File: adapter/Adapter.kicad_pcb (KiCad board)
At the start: 4 copper layers, 54 parts, among them J1 USB_B_Micro, J2 2040210-1, J3 USB_C_Receptacle, J4 Conn_01x05_Male, J5 Conn_01x03_Male, Q1 IRLML2244TRPBF, SW1 BOOT, SW2 BOOT, U1 SN75DP119RGYT, U2 LD1117S33TR, U3 STM32F072C8Tx, Y1 8MHZ

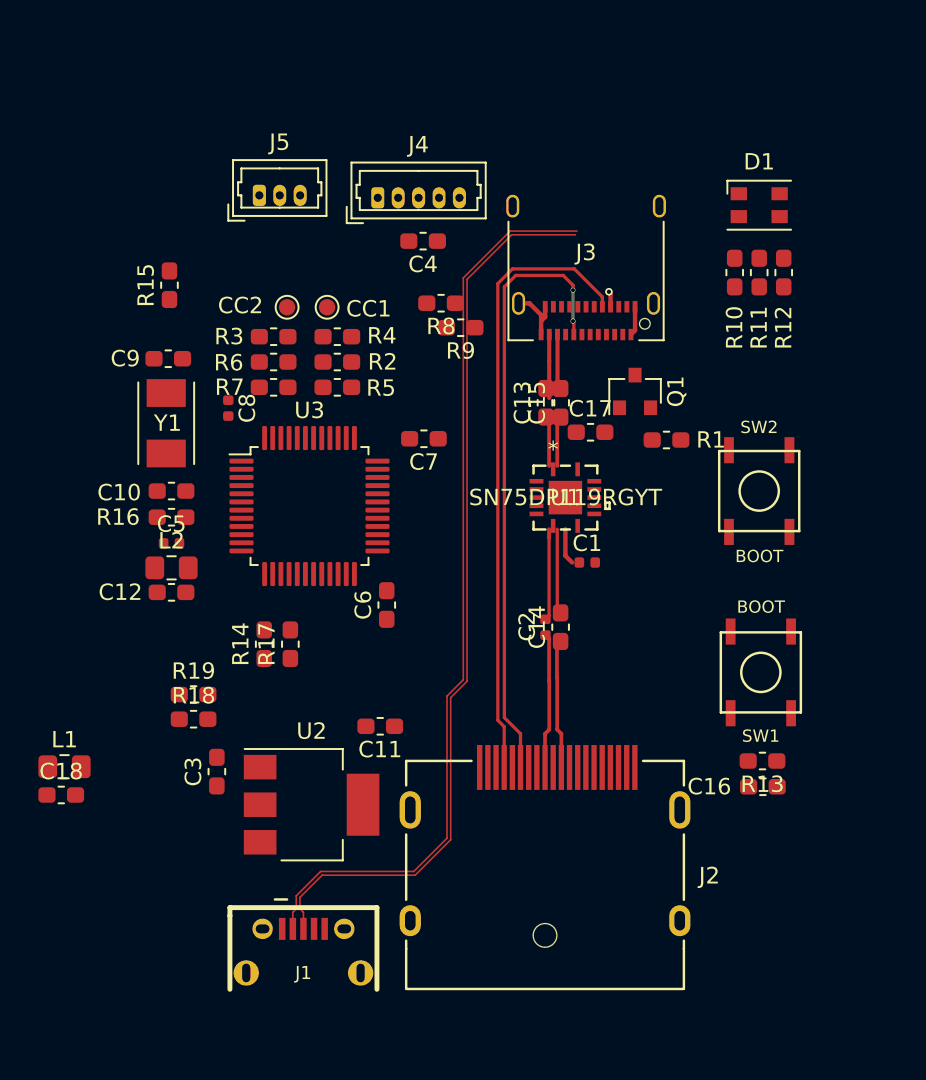
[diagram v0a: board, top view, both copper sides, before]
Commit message: placement mostly done
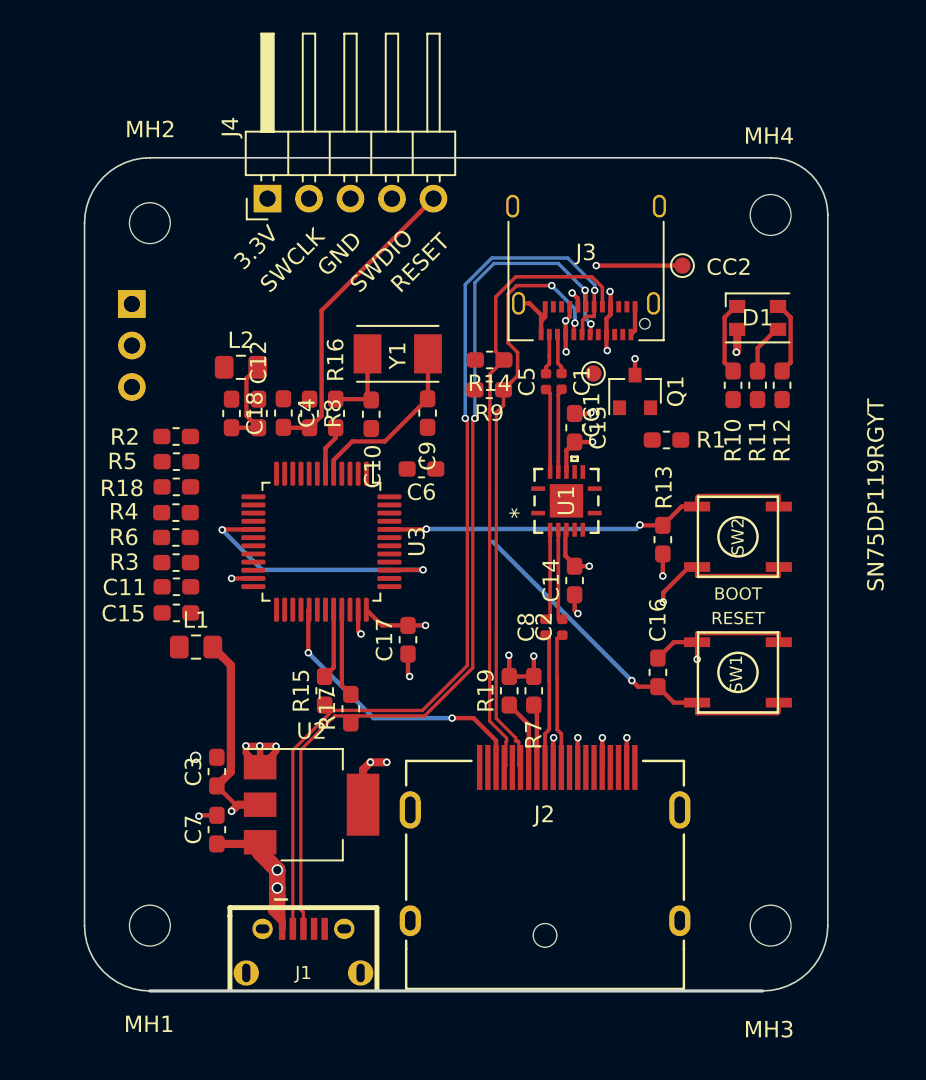
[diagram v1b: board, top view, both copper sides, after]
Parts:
- added MH1: MountingHole, MountingHole:MountingHole_2.5mm, F.Cu at (29.5, 80.0)
- added MH2: MountingHole, MountingHole:MountingHole_2.5mm, F.Cu at (29.5, 37.0)
- added MH3: MountingHole, MountingHole:MountingHole_2.5mm, F.Cu at (67.5, 80.0)
- added MH4: MountingHole, MountingHole:MountingHole_2.5mm, F.Cu at (67.5, 36.5)
- J4: footprint Connector_Molex:Molex_PicoBlade_53047-0510_1x05_P1.25mm_Vertical -> Connector_PinHeader_2.54mm:PinHeader_1x05_P2.54mm_Horizontal
- J5: footprint Connector_Molex:Molex_PicoBlade_53047-0310_1x03_P1.25mm_Vertical -> Connector_PinHeader_2.54mm:PinHeader_1x03_P2.54mm_Horizontal; moved to B.Cu
- R18: value 1M -> 97.6
- R5: value 100 -> 97.6
- R7: value 100 -> 1M
- SW1: value BOOT -> RESET
- U2: footprint Package_TO_SOT_SMD:SOT-223 -> Package_TO_SOT_SMD:SOT-223-3_TabPin2
- moved C7 27.1 mm to (33.6, 74.1), turned to 90 degrees
- moved C15 26.8 mm to (31.1, 60.9), turned to 0 degrees
- moved R15 26.6 mm to (40.2, 65.6)
- moved C18 25.6 mm to (34.5, 48.6), turned to 270 degrees
- moved C5 25.0 mm to (53.8, 46.7), turned to 90 degrees
- moved R7 24.5 mm to (53.0, 65.6), turned to 90 degrees
- moved CC2 24.3 mm to (62.1, 39.6), turned to 0 degrees
- moved C8 23.6 mm to (53.7, 61.7), turned to 90 degrees
- moved R14 22.2 mm to (50.3, 45.4), turned to 180 degrees
- moved R19 19.3 mm to (51.5, 65.6), turned to 90 degrees
- moved C17 16.9 mm to (45.3, 62.5), turned to 90 degrees
- moved CC1 16.8 mm to (56.6, 46.2), turned to 90 degrees
- moved C9 16.2 mm to (46.5, 48.6), turned to 270 degrees
- moved C11 15.1 mm to (31.1, 59.3), turned to 0 degrees
- moved R3 15.1 mm to (31.1, 57.8), turned to 180 degrees
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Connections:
- C1 pad 2: /DP_OUT_0+ -> /DP_OUT_0-
- C2 pad 1: /DP_IN_0+ -> /DP_IN_0-
- C5 pad 2: /DP_OUT_0- -> /DP_OUT_0+
- C8 pad 1: /DP_IN_0- -> /DP_IN_0+
- R18 pad 1: /CONFIG1 -> /CC2_TX
- R18 pad 2: GND -> /CC2
- R7 pad 1: /CC2_TX -> /CONFIG1
- R7 pad 2: /CC2 -> GND
- U3 pad 11: /CC1_RX -> EQ_CTL
- U3 pad 13: /CC2_RX -> VOD_CTL
- U3 pad 17: VOD_CTL -> /TX_CLK
- U3 pad 18: EQ_CTL -> /CC1_RX
- U3 pad 19: /TX_CLK -> /CC2_RX
- U3 pad 20: Net-(U3-Pad20) -> /CC2_EN
- U3 pad 42: /CC2_EN -> Net-(U3-Pad42)
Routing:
- net /nRESET: track 0.00 -> 41.6 mm, vias 0 -> 1
- net GND: track 12.8 -> 42.5 mm, vias 0 -> 18
- net /BOOT: track 0.00 -> 25.7 mm, vias 0 -> 2
- net +3V3: track 7.80 -> 32.4 mm, vias 0 -> 6
- net /HPD: track 0.00 -> 18.0 mm, vias 0 -> 2
- net /TX_CLK: track 0.00 -> 17.3 mm, vias 0 -> 2
- net VBUS: track 0.00 -> 11.1 mm, vias 0 -> 3
- net Net-(C9-Pad1): track 0.00 -> 10.9 mm
- net /CC2: track 0.00 -> 9.12 mm, vias 0 -> 2
- net Net-(J3-PadA4): track 0.96 -> 7.63 mm, vias 1 -> 5
- net VDDA: track 0.00 -> 5.94 mm
- net Net-(C8-Pad2): track 0.00 -> 5.48 mm
- net Net-(R17-Pad2): track 0.00 -> 5.42 mm
- net Net-(C5-Pad1): track 0.00 -> 5.15 mm
- net Net-(C1-Pad1): track 0.00 -> 5.14 mm
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- added copper zone on In2.Cu, net +3V3
- added copper zone on In1.Cu, net GND
- added copper zone on In2.Cu, net GND
- added copper zone on In2.Cu, net Net-(J3-PadA4)
- added copper zone on In2.Cu, net VBUS
- added copper zone on In2.Cu, net VDD
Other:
- board outline added: 45.5 x 51 mm
- board text added: "3.3V"
- board text added: "GND"
- board text added: "RESET"
- board text added: "SWCLK"
- board text added: "SWDIO"
